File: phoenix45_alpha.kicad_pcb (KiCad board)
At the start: 2 copper layers, 247.7 x 77.5 mm, 125 parts, among them J1 AVR-ISP-6, SW1 SW_PUSH, SW2 SW_PUSH, U1 SRV05-4, U2 ATmega32U4-M, U3 ATmega32U4-M, X1 Crystal_GND24_Small

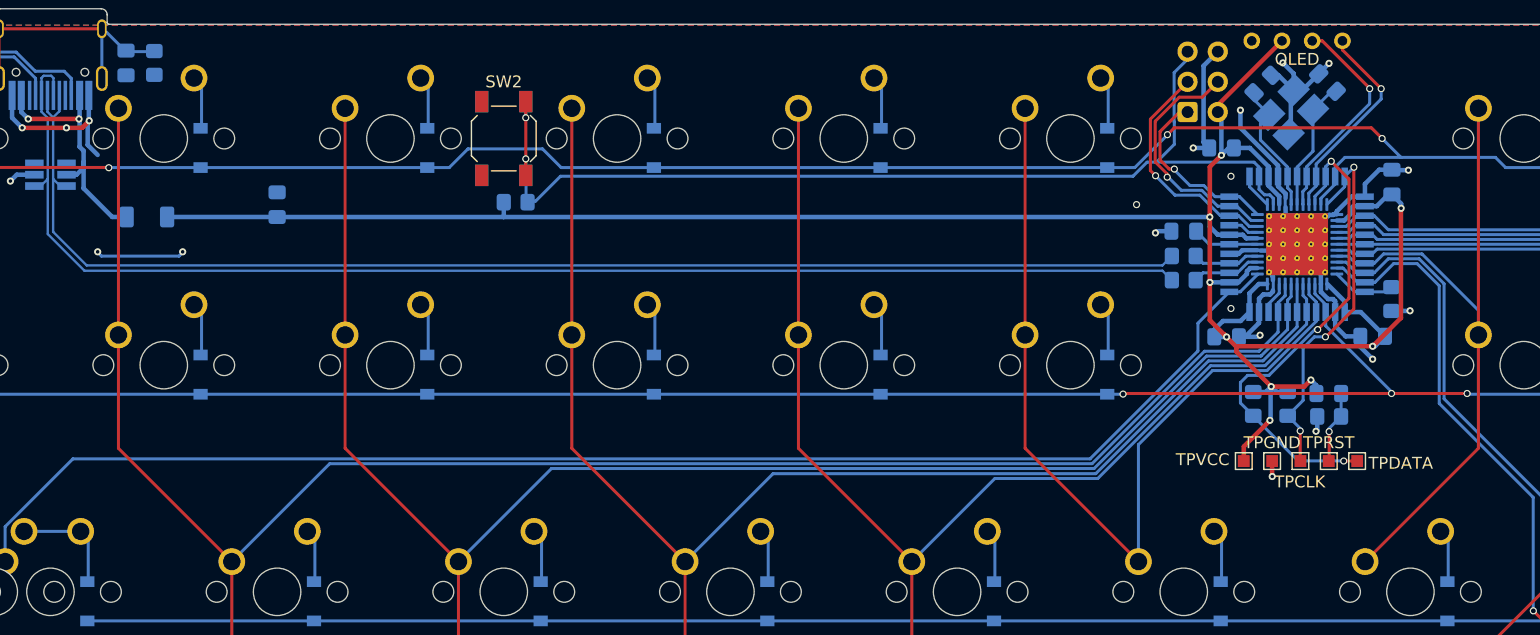
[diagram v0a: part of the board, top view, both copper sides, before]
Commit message: THT
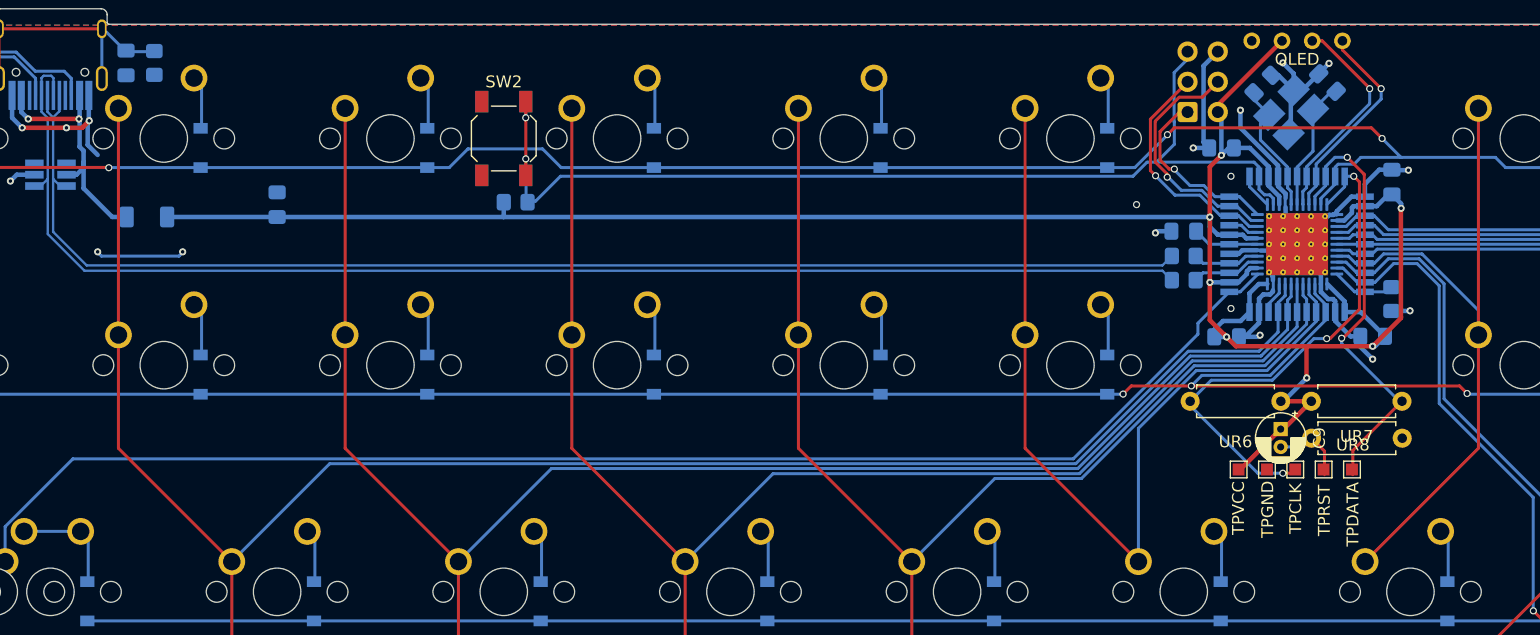
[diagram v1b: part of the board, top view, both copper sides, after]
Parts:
- C9: footprint Capacitor_SMD:C_0805_2012Metric_Pad1.18x1.45mm_HandSolder -> Capacitor_THT:CP_Radial_D4.0mm_P1.50mm; moved to F.Cu
- UR6, UR7, UR8: footprint Resistor_SMD:R_0805_2012Metric_Pad1.20x1.40mm_HandSolder -> Resistor_THT:R_Axial_DIN0207_L6.3mm_D2.5mm_P7.62mm_Horizontal; moved to F.Cu
- moved UR7 12.5 mm to (158.0, 59.4), turned to 180 degrees
- moved C9 5.03 mm to (147.8, 61.7), turned to -90 degrees
- moved UR8 2.35 mm to (150.4, 62.5), turned to 0 degrees
- moved TP1 0.83 mm to (149.1, 65.1)
- moved TP2 0.83 mm to (144.3, 65.1)
- moved TP3 0.83 mm to (146.7, 65.1)
- moved TP5 0.83 mm to (151.5, 65.1)
- moved TP4 0.83 mm to (153.8, 65.1)
- moved UR6 0.61 mm to (147.9, 59.4), turned to 180 degrees
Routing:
- net PD5: track 32.1 -> 43.7 mm
- net row1: track 240.5 -> 246.2 mm
- net PD2: track 42.0 -> 38.0 mm, vias 3 -> 2
- net +5V: track 204.0 -> 200.4 mm, vias 9 -> 7
- net GND: track 99.0 -> 96.1 mm, vias 20 -> 18
- net col0: track 163.2 -> 162.4 mm
- net col5: track 74.5 -> 75.3 mm
- net MISO: track 15.5 -> 14.8 mm
- net Net-(TP5-Pad1): track 6.11 -> 6.42 mm, vias 1 -> 0
